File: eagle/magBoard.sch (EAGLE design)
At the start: 9 parts, among them J1 RJ11-6PTH, U3 MAX3232PTH

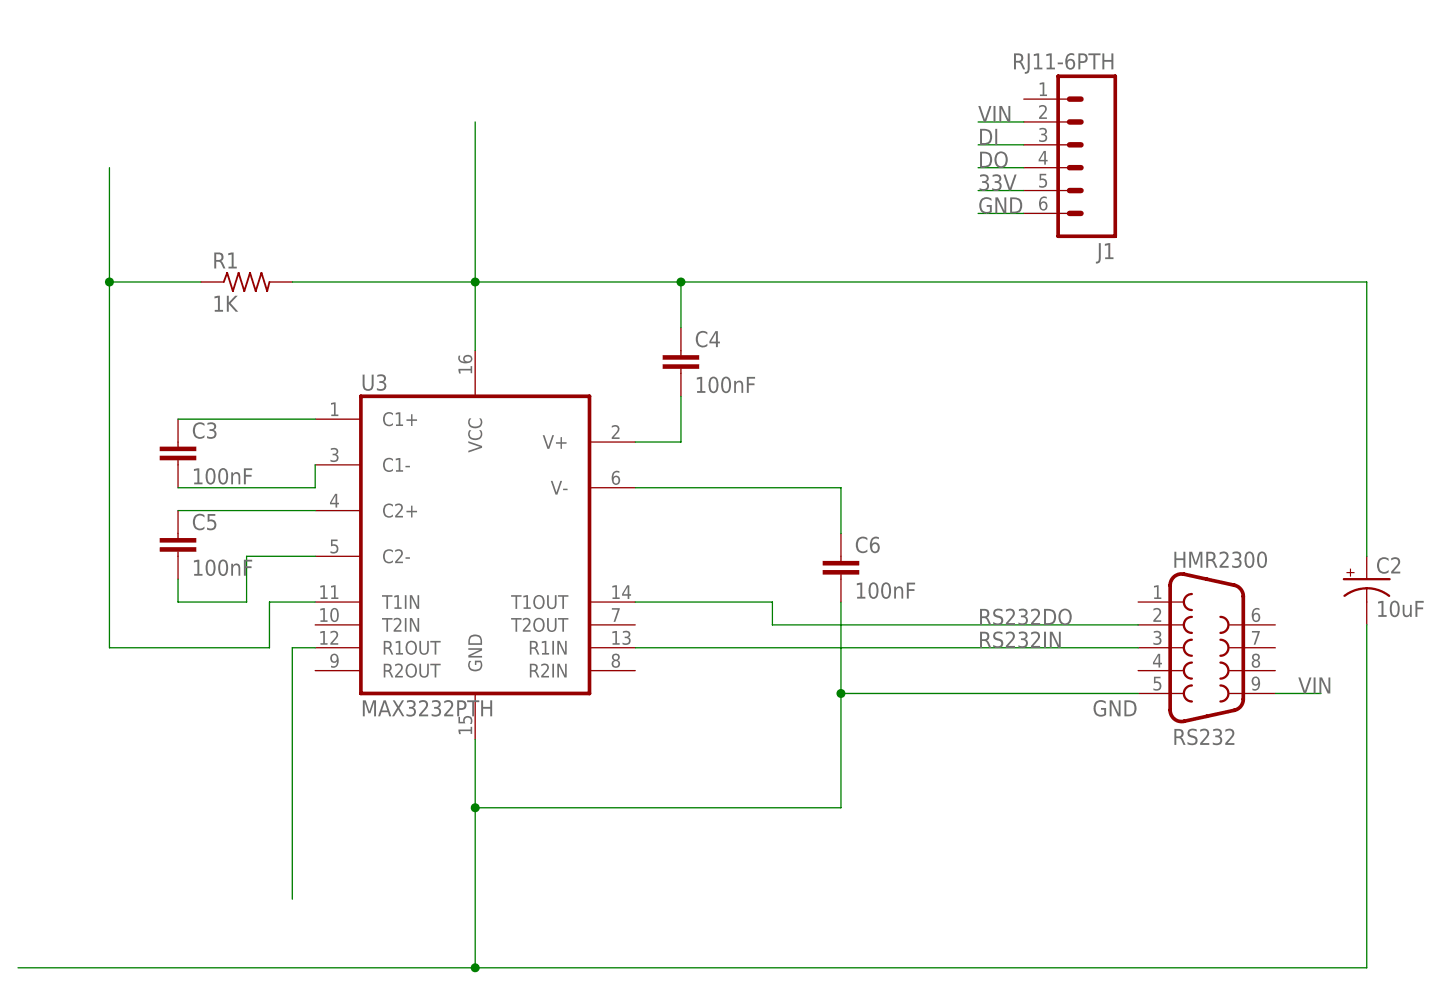
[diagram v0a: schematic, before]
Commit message: wrote a bunch and added references and pictures
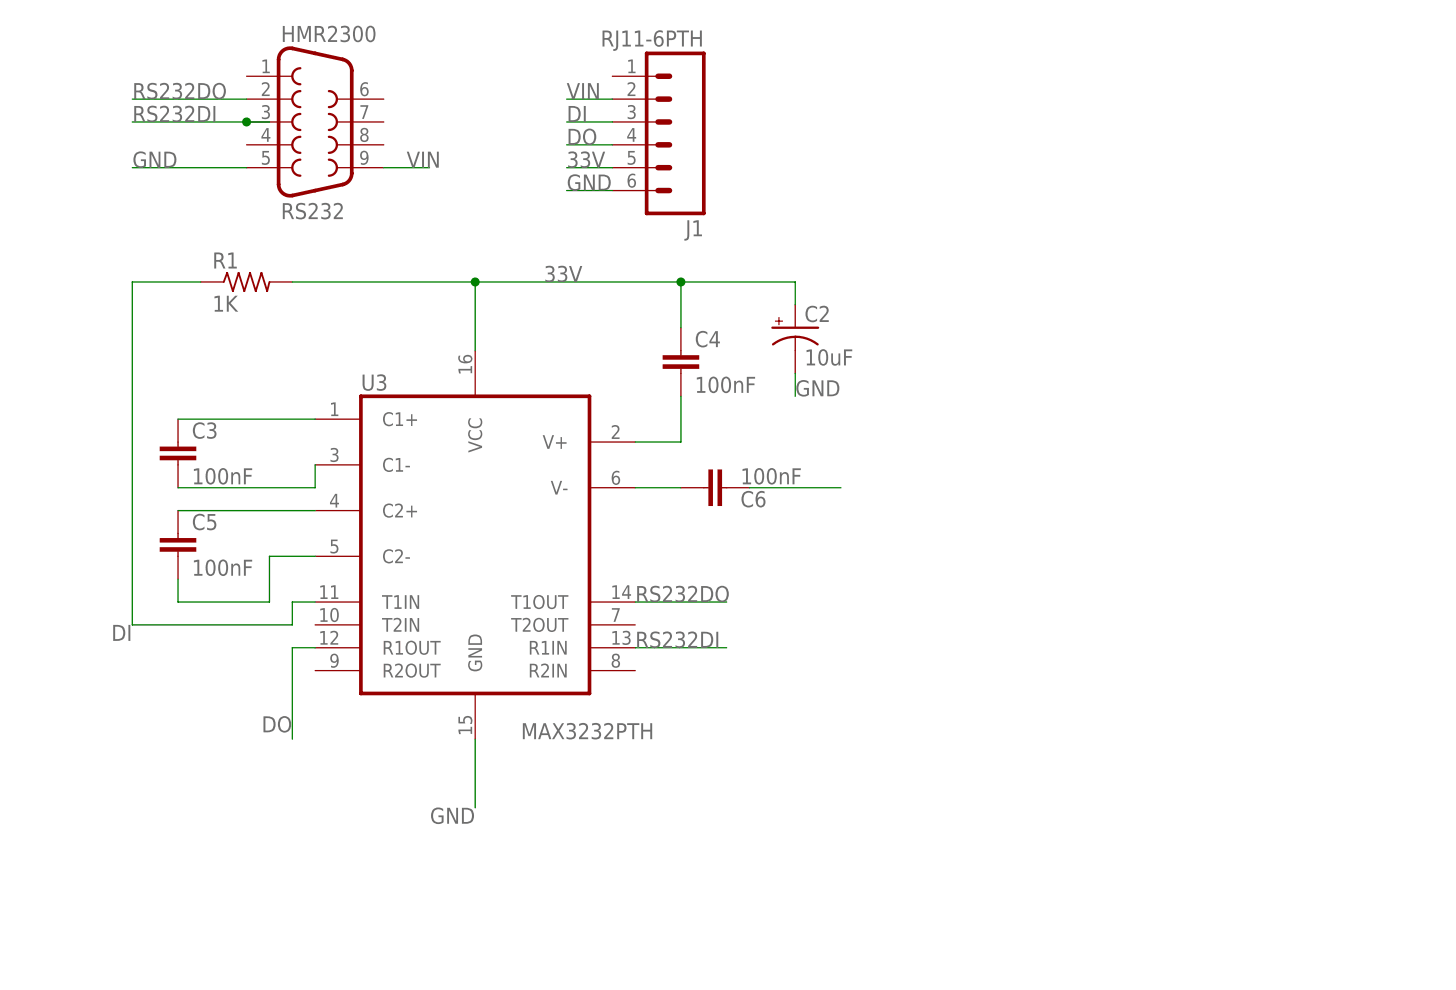
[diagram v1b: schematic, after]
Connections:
- net RS232IN renamed RS232DI
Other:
- moved on the sheet: C2, C6, HMR2300, J1
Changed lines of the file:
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@@
 </plain>
 <instances>
-<instance part="U3" gate="G$1" x="-2.54" y="0"/>
+<instance part="U3" gate="G$1" x="-2.54" y="0" smashed="yes">
+<attribute name="NAME" x="-12.7" y="15.875" size="1.778" layer="95"/>
+<attribute name="VALUE" x="5.08" y="-22.86" size="1.778" layer="96"/>
+</instance>
 <instance part="C4" gate="G$1" x="22.86" y="17.78"/>
 <instance part="C3" gate="G$1" x="-33.02" y="7.62"/>
 <instance part="C5" gate="G$1" x="-33.02" y="-2.54"/>
-<instance part="C6" gate="G$1" x="40.64" y="-5.08"/>
-<instance part="HMR2300" gate="G$1" x="81.28" y="-12.7"/>
-<instance part="J1" gate="G$1" x="66.04" y="43.18" rot="R180"/>
+<instance part="C6" gate="G$1" x="27.94" y="5.08" smashed="yes" rot="R90">
+<attribute name="NAME" x="29.464" y="2.921" size="1.778" layer="95"/>
+<attribute name="VALUE" x="29.464" y="5.461" size="1.778" layer="96"/>
+</instance>
+<instance part="HMR2300" gate="G$1" x="-17.78" y="45.72"/>
+<instance part="J1" gate="G$1" x="20.32" y="45.72" rot="R180"/>
 <instance part="R1" gate="G$1" x="-25.4" y="27.94"/>
-<instance part="C2" gate="G$1" x="99.06" y="-5.08"/>
+<instance part="C2" gate="G$1" x="35.56" y="22.86"/>
 </instances>
 <busses>
@@
 <segment>
 <pinref part="U3" gate="G$1" pin="C2-"/>
-<wire x1="-17.78" y1="-2.54" x2="-25.4" y2="-2.54" width="0.1524" layer="91"/>
-<wire x1="-25.4" y1="-2.54" x2="-25.4" y2="-7.62" width="0.1524" layer="91"/>
+<wire x1="-17.78" y1="-2.54" x2="-22.86" y2="-2.54" width="0.1524" layer="91"/>
+<wire x1="-22.86" y1="-2.54" x2="-22.86" y2="-7.62" width="0.1524" layer="91"/>
 <pinref part="C5" gate="G$1" pin="2"/>
-<wire x1="-25.4" y1="-7.62" x2="-33.02" y2="-7.62" width="0.1524" layer="91"/>
+<wire x1="-22.86" y1="-7.62" x2="-33.02" y2="-7.62" width="0.1524" layer="91"/>
 <wire x1="-33.02" y1="-7.62" x2="-33.02" y2="-5.08" width="0.1524" layer="91"/>
 </segment>
@@
 <wire x1="22.86" y1="27.94" x2="22.86" y2="22.86" width="0.1524" layer="91"/>
 <junction x="0" y="27.94"/>
-<wire x1="0" y1="45.72" x2="0" y2="27.94" width="0.1524" layer="91"/>
 <pinref part="R1" gate="G$1" pin="2"/>
 <wire x1="-20.32" y1="27.94" x2="0" y2="27.94" width="0.1524" layer="91"/>
 <pinref part="C2" gate="G$1" pin="+"/>
-<wire x1="22.86" y1="27.94" x2="99.06" y2="27.94" width="0.1524" layer="91"/>
-<wire x1="99.06" y1="27.94" x2="99.06" y2="-2.54" width="0.1524" layer="91"/>
+<wire x1="22.86" y1="27.94" x2="35.56" y2="27.94" width="0.1524" layer="91"/>
+<wire x1="35.56" y1="27.94" x2="35.56" y2="25.4" width="0.1524" layer="91"/>
 <junction x="22.86" y="27.94"/>
+<label x="7.62" y="27.94" size="1.778" layer="95"/>
 </segment>
 <segment>
 <pinref part="J1" gate="G$1" pin="5"/>
-<wire x1="60.96" y1="38.1" x2="55.88" y2="38.1" width="0.1524" layer="91"/>
-<label x="55.88" y="38.1" size="1.778" layer="95"/>
+<wire x1="15.24" y1="40.64" x2="10.16" y2="40.64" width="0.1524" layer="91"/>
+<label x="10.16" y="40.64" size="1.778" layer="95"/>
 </segment>
 </net>
@@
 <pinref part="U3" gate="G$1" pin="V-"/>
 <pinref part="C6" gate="G$1" pin="1"/>
-<wire x1="17.78" y1="5.08" x2="40.64" y2="5.08" width="0.1524" layer="91"/>
-<wire x1="40.64" y1="5.08" x2="40.64" y2="0" width="0.1524" layer="91"/>
+<wire x1="17.78" y1="5.08" x2="22.86" y2="5.08" width="0.1524" layer="91"/>
 </segment>
 </net>
 <net name="GND" class="0">
 <segment>
-<pinref part="U3" gate="G$1" pin="GND"/>
-<wire x1="0" y1="-22.86" x2="0" y2="-30.48" width="0.1524" layer="91"/>
-<wire x1="0" y1="-30.48" x2="40.64" y2="-30.48" width="0.1524" layer="91"/>
-<wire x1="40.64" y1="-30.48" x2="40.64" y2="-17.78" width="0.1524" layer="91"/>
-<pinref part="HMR2300" gate="G$1" pin="5"/>
-<wire x1="73.66" y1="-17.78" x2="40.64" y2="-17.78" width="0.1524" layer="91"/>
-<wire x1="0" y1="-30.48" x2="0" y2="-48.26" width="0.1524" layer="91"/>
-<junction x="0" y="-30.48"/>
-<wire x1="0" y1="-48.26" x2="-50.8" y2="-48.26" width="0.1524" layer="91"/>
-<pinref part="C2" gate="G$1" pin="-"/>
-<wire x1="99.06" y1="-10.16" x2="99.06" y2="-48.26" width="0.1524" layer="91"/>
-<wire x1="99.06" y1="-48.26" x2="0" y2="-48.26" width="0.1524" layer="91"/>
-<junction x="0" y="-48.26"/>
+<wire x1="40.64" y1="5.08" x2="30.48" y2="5.08" width="0.1524" layer="91"/>
 <pinref part="C6" gate="G$1" pin="2"/>
-<wire x1="40.64" y1="-7.62" x2="40.64" y2="-17.78" width="0.1524" layer="91"/>
-<junction x="40.64" y="-17.78"/>
-<label x="68.58" y="-20.32" size="1.778" layer="95"/>
 </segment>
 <segment>
 <pinref part="J1" gate="G$1" pin="6"/>
-<wire x1="60.96" y1="35.56" x2="55.88" y2="35.56" width="0.1524" layer="91"/>
-<label x="55.88" y="35.56" size="1.778" layer="95"/>
+<wire x1="15.24" y1="38.1" x2="10.16" y2="38.1" width="0.1524" layer="91"/>
+<label x="10.16" y="38.1" size="1.778" layer="95"/>
 </segment>
-</net>
-<net name="RS232IN" class="0">
 <segment>
-<pinref part="HMR2300" gate="G$1" pin="3"/>
-<pinref part="U3" gate="G$1" pin="R1IN"/>
-<wire x1="73.66" y1="-12.7" x2="17.78" y2="-12.7" width="0.1524" layer="91"/>
-<label x="55.88" y="-12.7" size="1.778" layer="95"/>
+<pinref part="C2" gate="G$1" pin="-"/>
+<wire x1="35.56" y1="17.78" x2="35.56" y2="15.24" width="0.1524" layer="91"/>
+<label x="35.56" y="15.24" size="1.778" layer="95"/>
+</segment>
+<segment>
+<pinref part="HMR2300" gate="G$1" pin="5"/>
+<wire x1="-25.4" y1="40.64" x2="-38.1" y2="40.64" width="0.1524" layer="91"/>
+<label x="-38.1" y="40.64" size="1.778" layer="95"/>
+</segment>
+<segment>
+<pinref part="U3" gate="G$1" pin="GND"/>
+<wire x1="0" y1="-22.86" x2="0" y2="-30.48" width="0.1524" layer="91"/>
+<label x="0" y="-30.48" size="1.778" layer="95" rot="R180"/>
 </segment>
 </net>
@@
 <segment>
 <pinref part="HMR2300" gate="G$1" pin="2"/>
-<wire x1="73.66" y1="-10.16" x2="33.02" y2="-10.16" width="0.1524" layer="91"/>
-<wire x1="33.02" y1="-10.16" x2="33.02" y2="-7.62" width="0.1524" layer="91"/>
+<wire x1="-25.4" y1="48.26" x2="-38.1" y2="48.26" width="0.1524" layer="91"/>
+<label x="-38.1" y="48.26" size="1.778" layer="95"/>
+</segment>
+<segment>
 <pinref part="U3" gate="G$1" pin="T1OUT"/>
-<wire x1="33.02" y1="-7.62" x2="17.78" y2="-7.62" width="0.1524" layer="91"/>
-<label x="55.88" y="-10.16" size="1.778" layer="95"/>
+<wire x1="27.94" y1="-7.62" x2="17.78" y2="-7.62" width="0.1524" layer="91"/>
+<label x="17.78" y="-7.62" size="1.778" layer="95"/>
 </segment>
 </net>
@@
 <pinref part="U3" gate="G$1" pin="R1OUT"/>
 <wire x1="-17.78" y1="-12.7" x2="-20.32" y2="-12.7" width="0.1524" layer="91"/>
-<wire x1="-20.32" y1="-12.7" x2="-20.32" y2="-40.64" width="0.1524" layer="91"/>
+<wire x1="-20.32" y1="-12.7" x2="-20.32" y2="-22.86" width="0.1524" layer="91"/>
+<label x="-20.32" y="-20.32" size="1.778" layer="95" rot="R180"/>
 </segment>
 <segment>
 <pinref part="J1" gate="G$1" pin="4"/>
-<wire x1="60.96" y1="40.64" x2="55.88" y2="40.64" width="0.1524" layer="91"/>
-<label x="55.88" y="40.64" size="1.778" layer="95"/>
+<wire x1="15.24" y1="43.18" x2="10.16" y2="43.18" width="0.1524" layer="91"/>
+<label x="10.16" y="43.18" size="1.778" layer="95"/>
 </segment>
 </net>
@@
 <segment>
 <pinref part="U3" gate="G$1" pin="T1IN"/>
-<wire x1="-17.78" y1="-7.62" x2="-22.86" y2="-7.62" width="0.1524" layer="91"/>
-<wire x1="-22.86" y1="-7.62" x2="-22.86" y2="-12.7" width="0.1524" layer="91"/>
-<wire x1="-22.86" y1="-12.7" x2="-40.64" y2="-12.7" width="0.1524" layer="91"/>
-<wire x1="-40.64" y1="40.64" x2="-40.64" y2="27.94" width="0.1524" layer="91"/>
+<wire x1="-17.78" y1="-7.62" x2="-20.32" y2="-7.62" width="0.1524" layer="91"/>
+<wire x1="-20.32" y1="-7.62" x2="-20.32" y2="-10.16" width="0.1524" layer="91"/>
+<wire x1="-20.32" y1="-10.16" x2="-38.1" y2="-10.16" width="0.1524" layer="91"/>
 <pinref part="R1" gate="G$1" pin="1"/>
-<wire x1="-40.64" y1="27.94" x2="-40.64" y2="-12.7" width="0.1524" layer="91"/>
-<wire x1="-40.64" y1="27.94" x2="-30.48" y2="27.94" width="0.1524" layer="91"/>
-<junction x="-40.64" y="27.94"/>
+<wire x1="-38.1" y1="27.94" x2="-38.1" y2="-10.16" width="0.1524" layer="91"/>
+<wire x1="-38.1" y1="27.94" x2="-30.48" y2="27.94" width="0.1524" layer="91"/>
+<label x="-38.1" y="-10.16" size="1.778" layer="95" rot="R180"/>
 </segment>
 <segment>
 <pinref part="J1" gate="G$1" pin="3"/>
-<wire x1="60.96" y1="43.18" x2="55.88" y2="43.18" width="0.1524" layer="91"/>
-<label x="55.88" y="43.18" size="1.778" layer="95"/>
+<wire x1="15.24" y1="45.72" x2="10.16" y2="45.72" width="0.1524" layer="91"/>
+<label x="10.16" y="45.72" size="1.778" layer="95"/>
 </segment>
 </net>
@@
 <segment>
 <pinref part="HMR2300" gate="G$1" pin="9"/>
-<wire x1="88.9" y1="-17.78" x2="93.98" y2="-17.78" width="0.1524" layer="91"/>
-<label x="91.44" y="-17.78" size="1.778" layer="95"/>
+<wire x1="-10.16" y1="40.64" x2="-5.08" y2="40.64" width="0.1524" layer="91"/>
+<label x="-7.62" y="40.64" size="1.778" layer="95"/>
 </segment>
 <segment>
 <pinref part="J1" gate="G$1" pin="2"/>
-<wire x1="60.96" y1="45.72" x2="55.88" y2="45.72" width="0.1524" layer="91"/>
-<label x="55.88" y="45.72" size="1.778" layer="95"/>
+<wire x1="15.24" y1="48.26" x2="10.16" y2="48.26" width="0.1524" layer="91"/>
+<label x="10.16" y="48.26" size="1.778" layer="95"/>
 </segment>
 </net>
+<net name="RS232DI" class="0">
+<segment>
+<pinref part="U3" gate="G$1" pin="R1IN"/>
+<wire x1="17.78" y1="-12.7" x2="27.94" y2="-12.7" width="0.1524" layer="91"/>
+<label x="17.78" y="-12.7" size="1.778" layer="95"/>
+</segment>
+<segment>
+<wire x1="-22.86" y1="45.72" x2="-25.4" y2="45.72" width="0.1524" layer="91"/>
+<label x="-38.1" y="45.72" size="1.778" layer="95"/>
+<pinref part="HMR2300" gate="G$1" pin="3"/>
+<wire x1="-25.4" y1="45.72" x2="-38.1" y2="45.72" width="0.1524" layer="91"/>
+<junction x="-25.4" y="45.72"/>
+</segment>
+</net>
